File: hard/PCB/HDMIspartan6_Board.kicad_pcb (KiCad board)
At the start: 4 copper layers, 56.1 x 89.6 mm, 150 parts, among them IC1 W9812G6KH, P1 CONN_02X20, P2 CONN_01X03, U1 XC6SLX9-2TQG144C, U2 TPS62133RGTR, U3 ZLDO1117G33TA, U4 ZLDO1117G12TA, U5 MAX5864

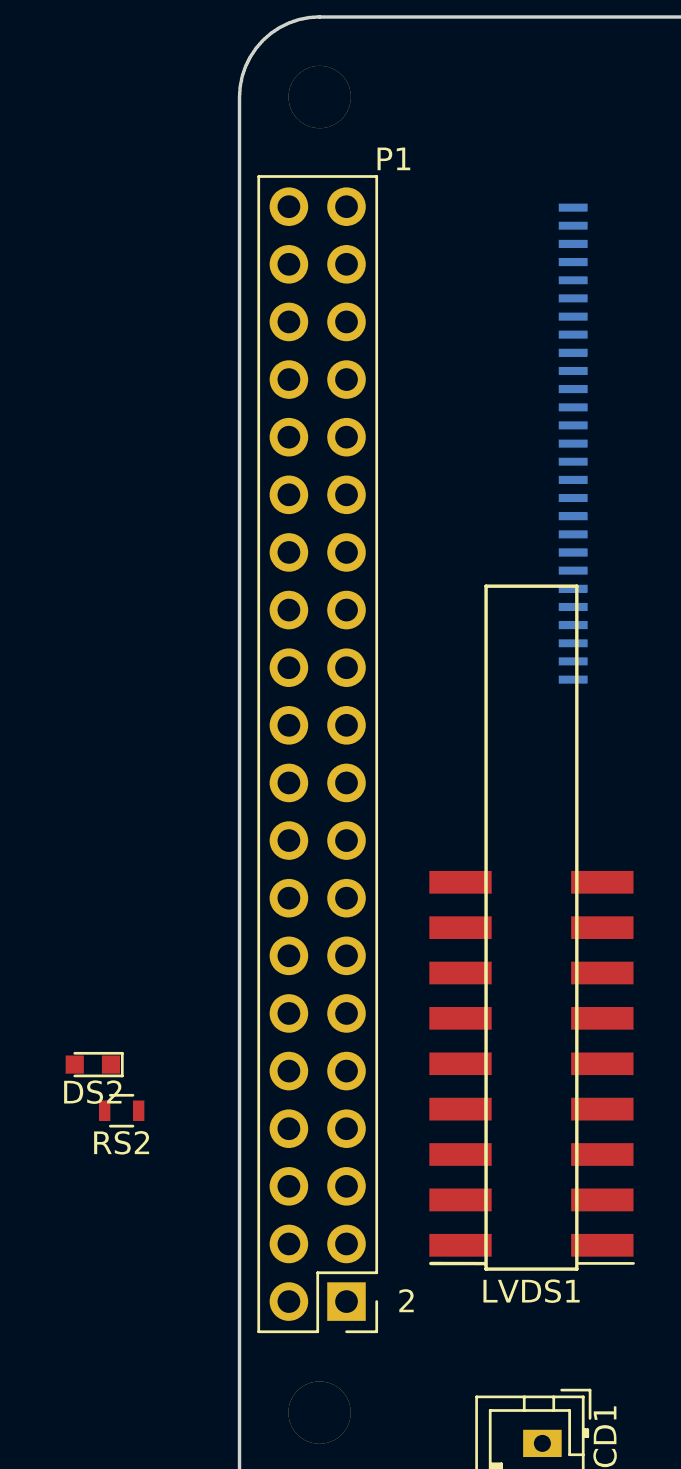
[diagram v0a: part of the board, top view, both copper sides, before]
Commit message: Test LVDS RAM
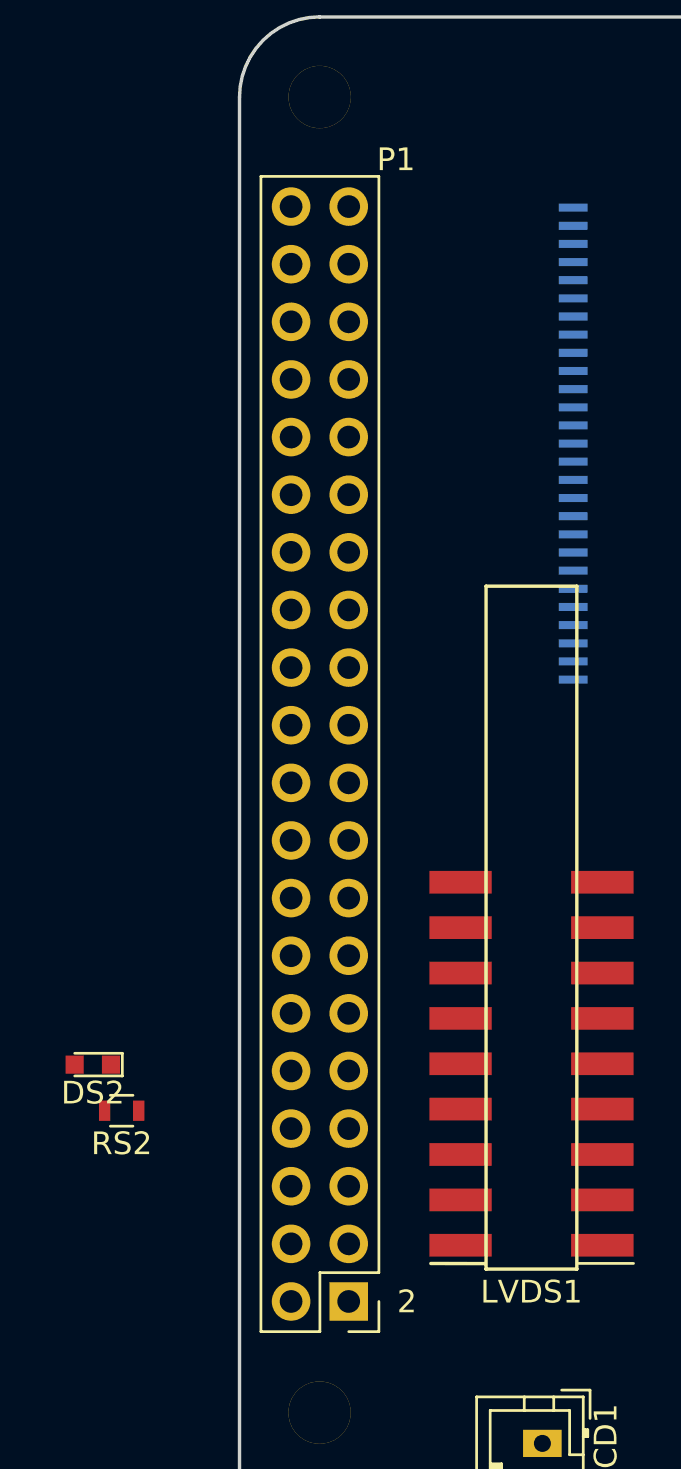
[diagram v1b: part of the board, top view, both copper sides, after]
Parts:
- moved P1 0.10 mm to (111.9, 66.7)
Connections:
- P1 pad 1: +3V3 -> Net-(P1-Pad1)
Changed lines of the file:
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@@
 (kicad_pcb (version 4) (host pcbnew 4.0.6-e0-6349~53~ubuntu16.04.1)
   (general
-    (links 435)
-    (no_connects 413)
+    (links 434)
+    (no_connects 412)
     (area 108.230759 59.595899 164.453801 149.311381)
     (thickness 1.6)
@@
     (zones 0)
     (modules 150)
-    (nets 234)
+    (nets 235)
   )
   (page A4)
@@
   (net 232 "Net-(RS2-Pad2)")
   (net 233 "Net-(S1-Pad1)")
+  (net 234 "Net-(P1-Pad1)")
   (net_class Default "This is the default net class."
     (clearance 0.15)
@@
     (add_net "Net-(JMS1-Pad4)")
     (add_net "Net-(L1-Pad2)")
+    (add_net "Net-(P1-Pad1)")
     (add_net "Net-(P1-Pad11)")
     (add_net "Net-(P1-Pad12)")
@@
   )
   (module Pin_Headers:Pin_Header_Straight_2x20_Pitch2.54mm locked (layer F.Cu)
-    (at 111.83128 66.69908 180)
+    (at 111.9278 66.694 180)
     (descr "Through hole straight pin header, 2x20, 2.54mm pitch, double rows")
     (tags "Through hole pin header THT 2x20 2.54mm double row")
@@
     )
     (pad 1 thru_hole rect (at -1.19126 -49.59858 180) (size 1.7 1.7) (drill 1) (layers *.Cu *.Mask)
-      (net 13 +3V3))
+      (net 234 "Net-(P1-Pad1)"))
     (pad 2 thru_hole oval (at 1.34874 -49.59858 180) (size 1.7 1.7) (drill 1) (layers *.Cu *.Mask)
       (net 50 VDD5V))
